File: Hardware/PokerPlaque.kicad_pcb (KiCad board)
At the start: 2 copper layers, 36.5 x 40.5 mm, 10 parts, among them J1 A2541WR-5P, J2 A2541WR-4P, J3 A2541WR-2P, J4 A2541WR-8P, SW1 KH-6X6X6H-STM, U1 CH32V203C8T6

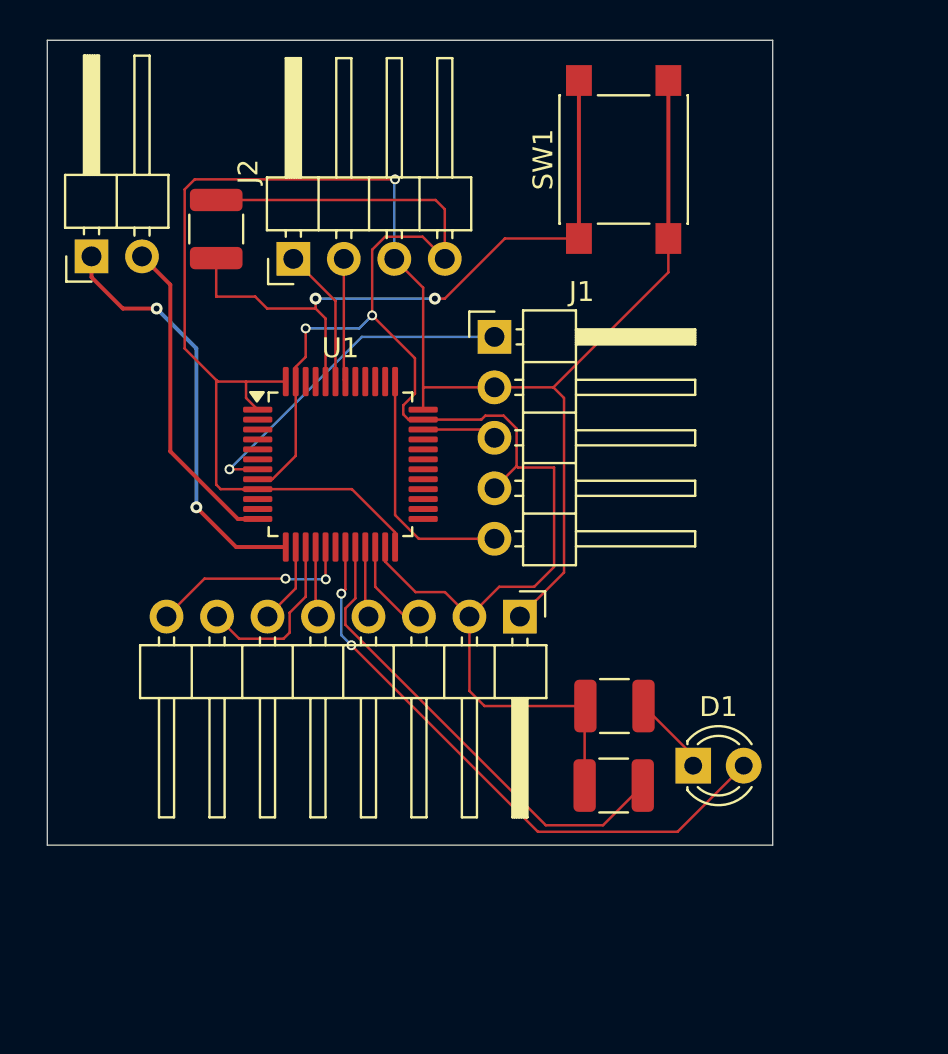
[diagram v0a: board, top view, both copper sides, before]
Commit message: feat: revamped
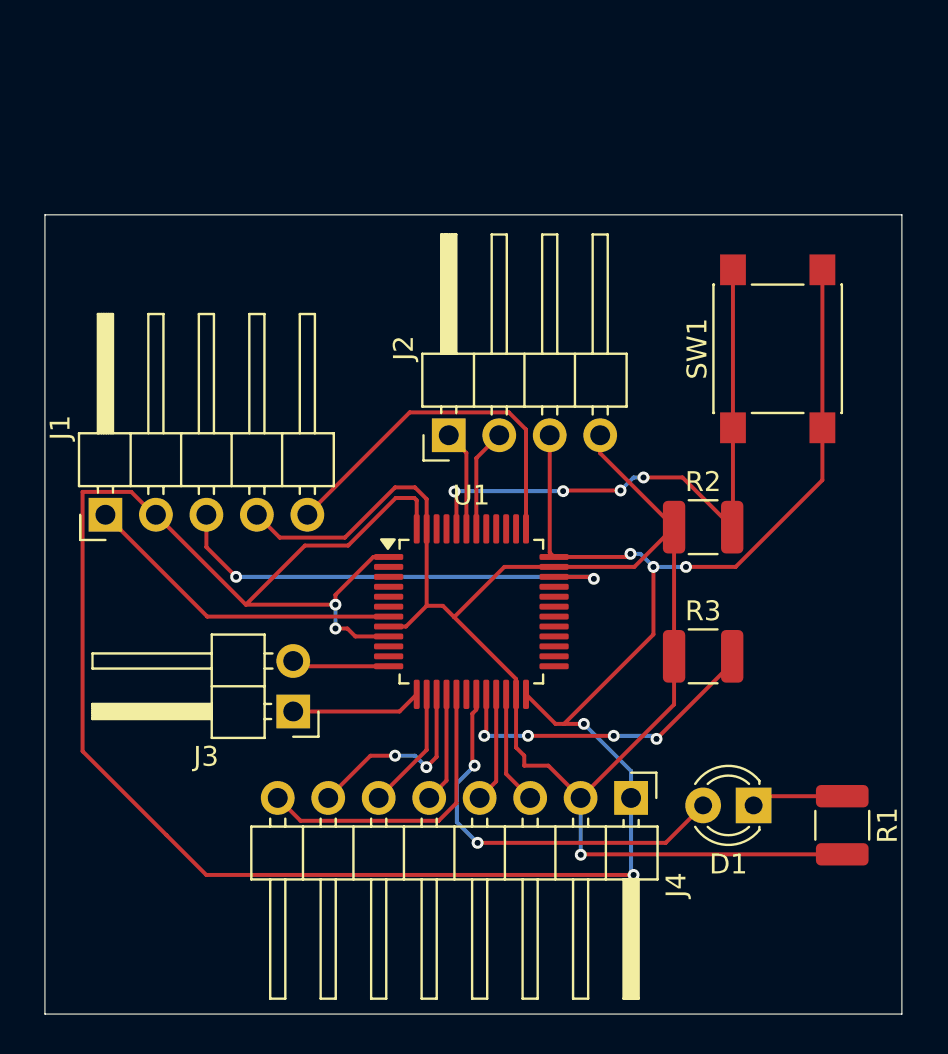
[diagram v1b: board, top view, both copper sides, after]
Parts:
- moved R2 28.7 mm to (55.0, 44.5), turned to 0 degrees
- moved J3 25.0 mm to (34.4, 53.8), turned to 180 degrees
- moved J1 21.5 mm to (24.9, 43.9), turned to 90 degrees
- moved R1 12.9 mm to (62.0, 59.5), turned to -90 degrees
- moved SW1 12.3 mm to (58.8, 35.5)
- moved J2 11.8 mm to (42.2, 39.9)
- moved J4 10.7 mm to (51.4, 58.1)
- moved U1 9.92 mm to (43.3, 48.8)
- moved R3 7.91 mm to (55.0, 51.0)
- moved D1 3.64 mm to (57.5, 58.5), turned to 180 degrees
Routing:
- net +3.3V: track 91.5 -> 133.1 mm, vias 1 -> 7
- net SWDIO: track 3.76 -> 23.8 mm, vias 0 -> 2
- net RESERVED_UART_RX: track 21.1 -> 6.57 mm, vias 2 -> 0
- net RESERVED_UART_TX: track 16.2 -> 4.91 mm
- net DEBUG_LED0: track 30.2 -> 20.5 mm
- net BOOT1: track 24.1 -> 16.6 mm, vias 0 -> 4
- net SWCLK: track 12.2 -> 18.5 mm
- net DISPLAY_MOSI1: track 10.5 -> 15.3 mm, vias 2 -> 0
- net BOOT0: track 34.0 -> 30.2 mm, vias 2 -> 4
- net DISPLAY_SS1: track 4.09 -> 6.21 mm
- net DISPLAY_MISO1: track 3.55 -> 5.57 mm
- net DISPLAY_RESET: track 3.57 -> 5.56 mm
- net I2C1_SDA: track 7.05 -> 5.08 mm
- net RST: track 17.5 -> 16.4 mm, vias 1 -> 0
- net DISPLAY_SCK1: track 8.88 -> 9.93 mm, vias 0 -> 2
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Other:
- board size 36.5 x 40.5 mm -> 43.1 x 40.2 mm
